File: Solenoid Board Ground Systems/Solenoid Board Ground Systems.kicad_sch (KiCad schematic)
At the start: 31 parts, among them J1 OUT CHAN 1, J2 CHAN IN, J3 OUT CHAN 2

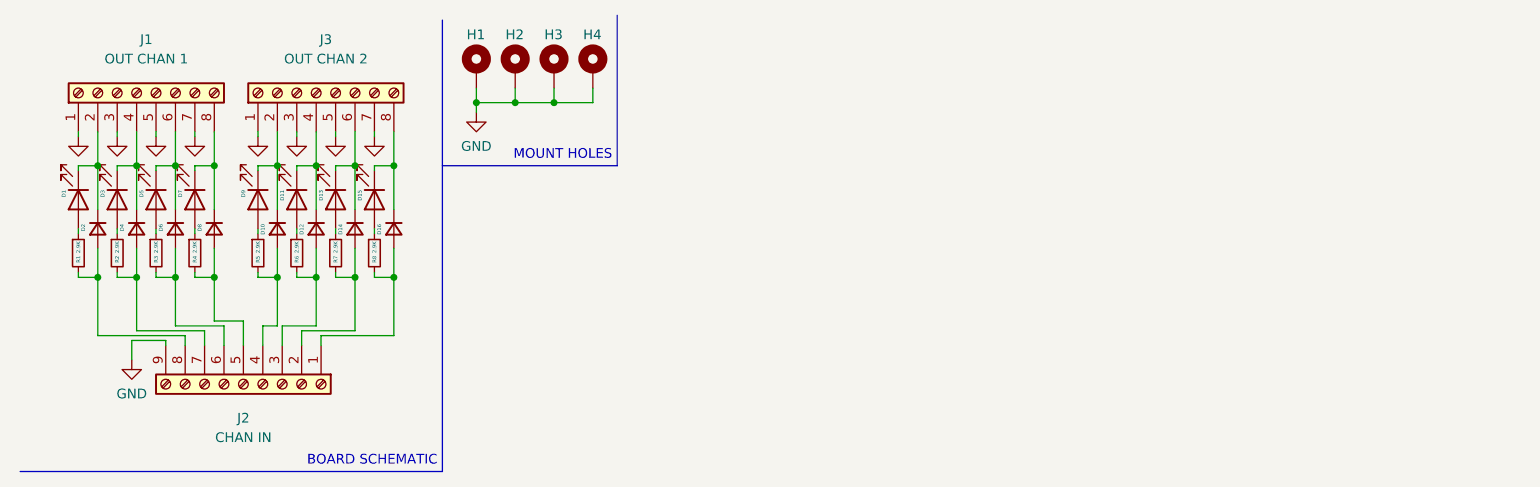
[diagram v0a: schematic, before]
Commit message: Ground System Work
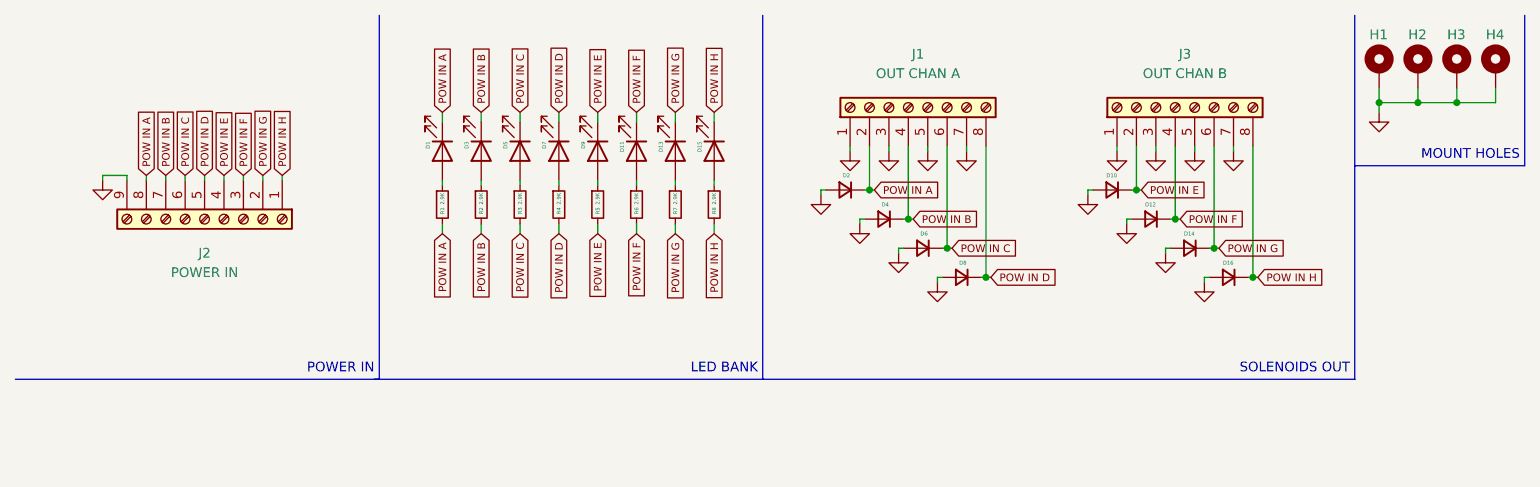
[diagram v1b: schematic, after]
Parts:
- J1: value OUT CHAN 1 -> OUT CHAN A
- J2: value CHAN IN -> POWER IN
- J3: value OUT CHAN 2 -> OUT CHAN B
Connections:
- net GND: now also D10.2 (A), D12.2 (A), D14.2 (A), D16.2 (A), D2.2 (A), D4.2 (A), D6.2 (A), D8.2 (A)
- net POW IN E: now reaches D10.1 (K), D9.1 (K), J3.2 (Pin_2)
- net POW IN E: now also J2.4 (Pin_4), R5.2
- net POW IN F: now reaches D11.1 (K), D12.1 (K), J3.4 (Pin_4)
- net POW IN F: now also J2.3 (Pin_3), R6.2
- net POW IN G: now reaches D13.1 (K), D14.1 (K), J3.6 (Pin_6)
- net POW IN G: now also J2.2 (Pin_2), R7.2
- net POW IN H: now reaches D15.1 (K), D16.1 (K), J3.8 (Pin_8)
- net POW IN H: now also J2.1 (Pin_1), R8.2
- net POW IN D: now reaches J2.5 (Pin_5), R4.2
- net POW IN D: now also D7.1 (K), D8.1 (K), J1.8 (Pin_8); no longer D8.2 (A)
- net POW IN C: now reaches J2.6 (Pin_6), R3.2
- net POW IN C: now also D5.1 (K), D6.1 (K), J1.6 (Pin_6); no longer D6.2 (A)
- net POW IN B: now reaches J2.7 (Pin_7), R2.2
- net POW IN B: now also D3.1 (K), D4.1 (K), J1.4 (Pin_4); no longer D4.2 (A)
- net POW IN A: now reaches J2.8 (Pin_8), R1.2
- net POW IN A: now also D1.1 (K), D2.1 (K), J1.2 (Pin_2); no longer D2.2 (A)
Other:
- note added: "LED BANK"
- note added: "POWER IN"
- note added: "SOLENOIDS OUT"
- note removed: "BOARD SCHEMATIC"
- moved on the sheet: D1, D10, D11, D12, D13, D14, D15, D16, D2, D3, D4, D5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
